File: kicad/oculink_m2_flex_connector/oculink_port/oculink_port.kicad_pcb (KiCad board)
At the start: 4 copper layers, 20.8 x 32.9 mm, 6 parts, among them J1 G14A42121B12HR, J2 Conn_01x38_Pin

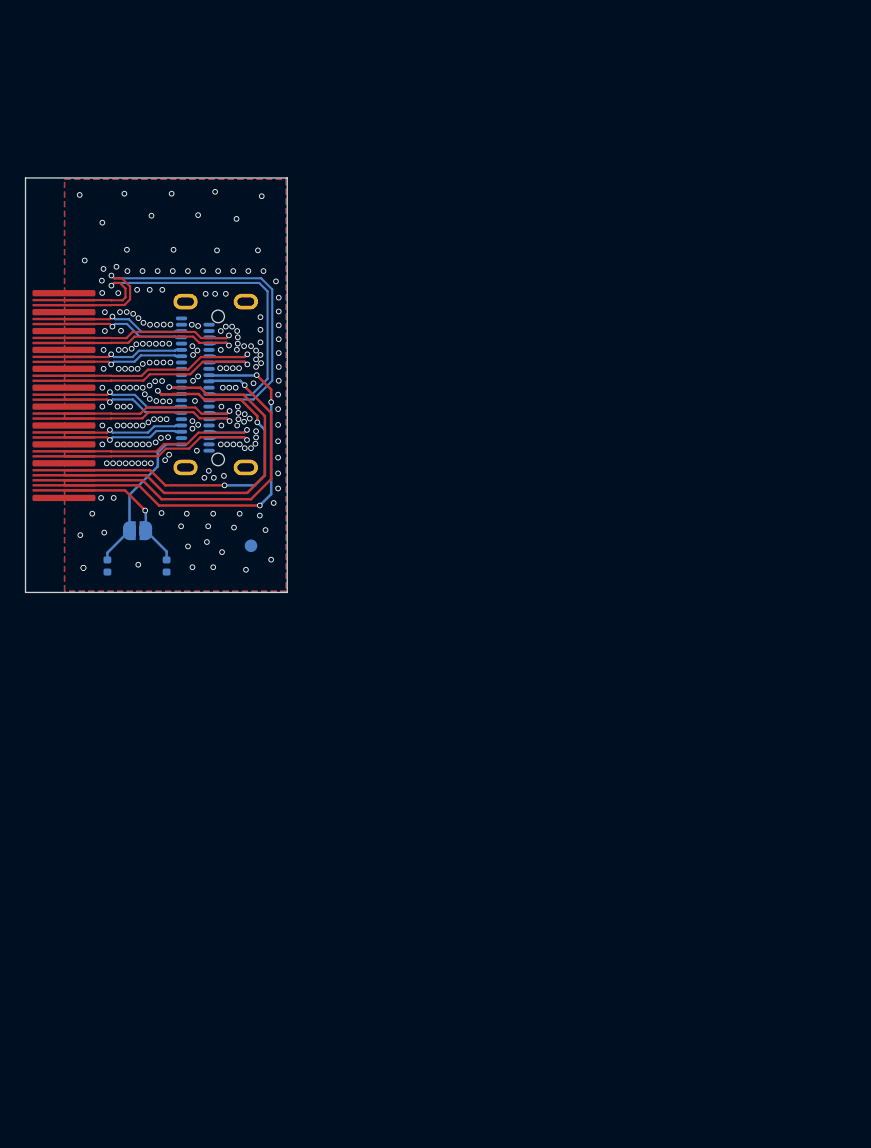
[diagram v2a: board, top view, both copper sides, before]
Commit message: Added mounting for port
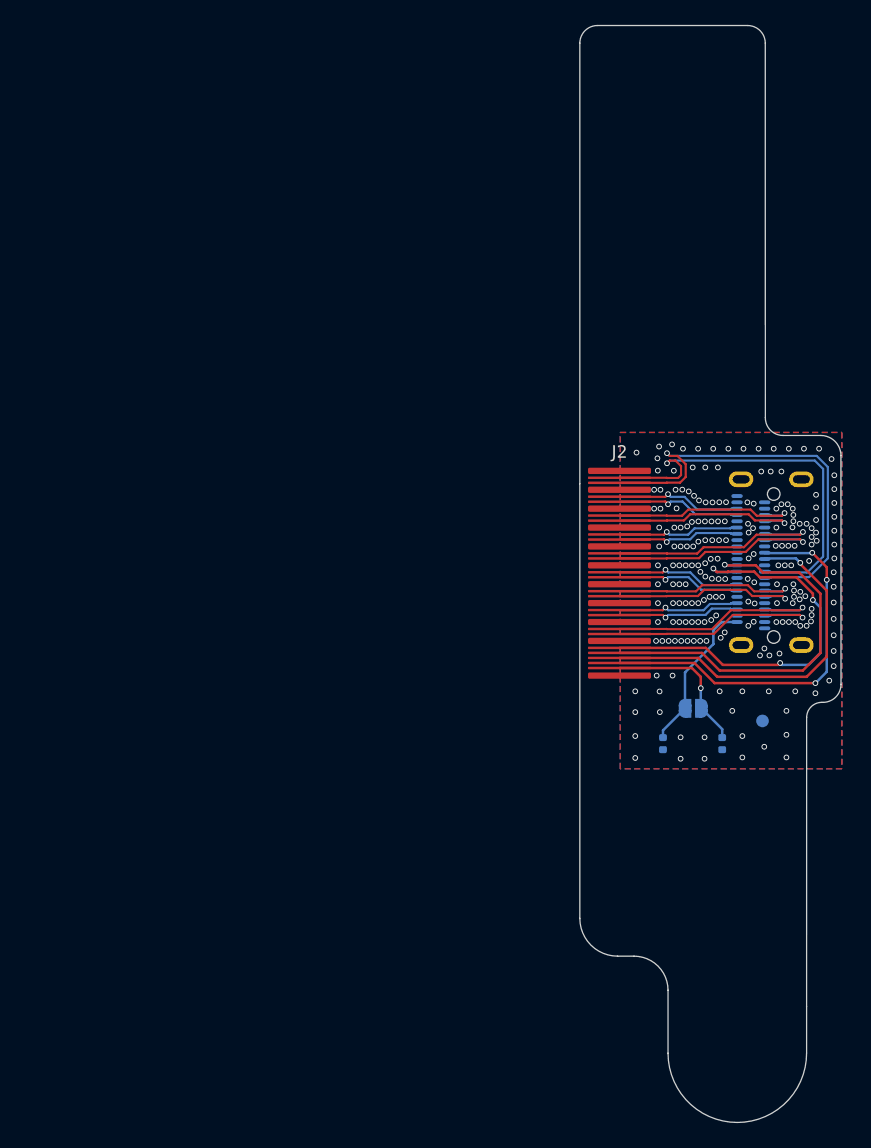
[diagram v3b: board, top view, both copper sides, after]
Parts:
- added ?: , , F.Cu at (187.1, 68.8)
- added ?: , , F.Cu at (192.2, 145.6)
- moved C1 46.3 mm to (186.3, 121.0)
- moved C5 46.3 mm to (191.0, 121.0)
- moved J1 46.3 mm to (195.1, 106.6)
- moved J2 46.3 mm to (182.8, 94.5)
- moved JP1 46.3 mm to (188.7, 118.2)
- moved TP2 42.9 mm to (194.2, 119.2)
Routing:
- net 3.3V_OPT: track 11.7 -> 12.3 mm
- net GND: vias 215 -> 205
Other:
- board size 20.8 x 32.9 mm -> 20.7 x 87.1 mm

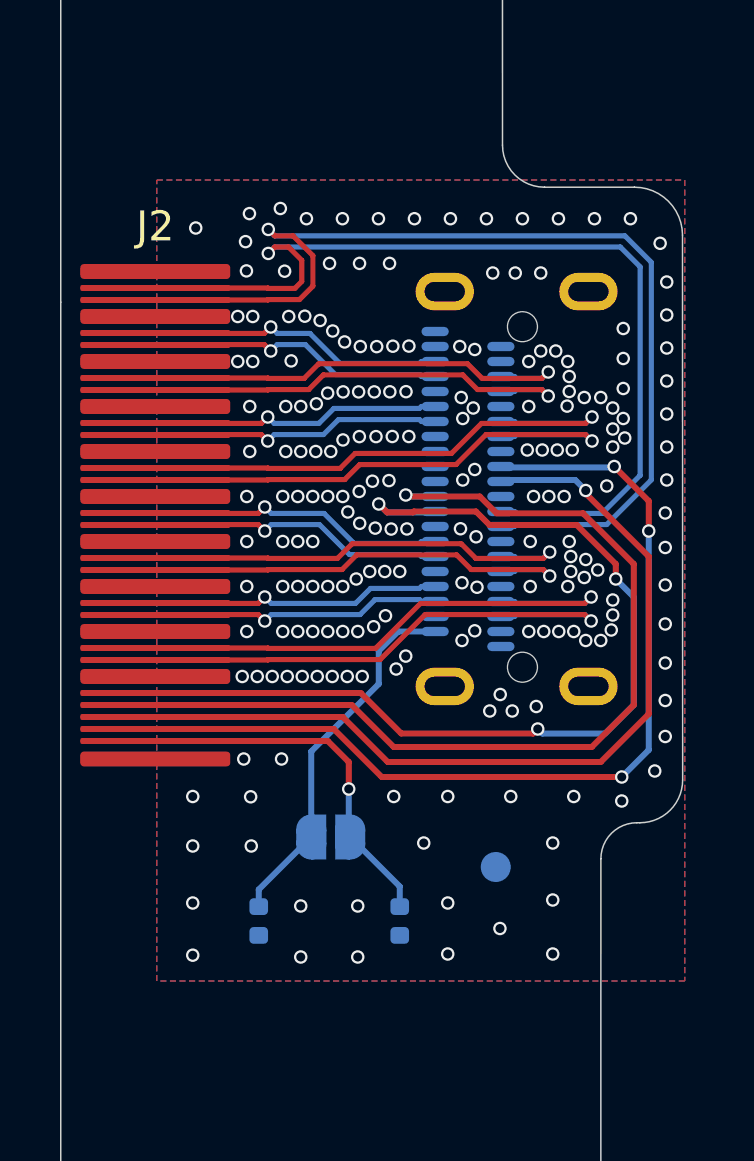
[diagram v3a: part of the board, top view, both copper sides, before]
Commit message: Shifted location of ffc connector to avoid screw mount
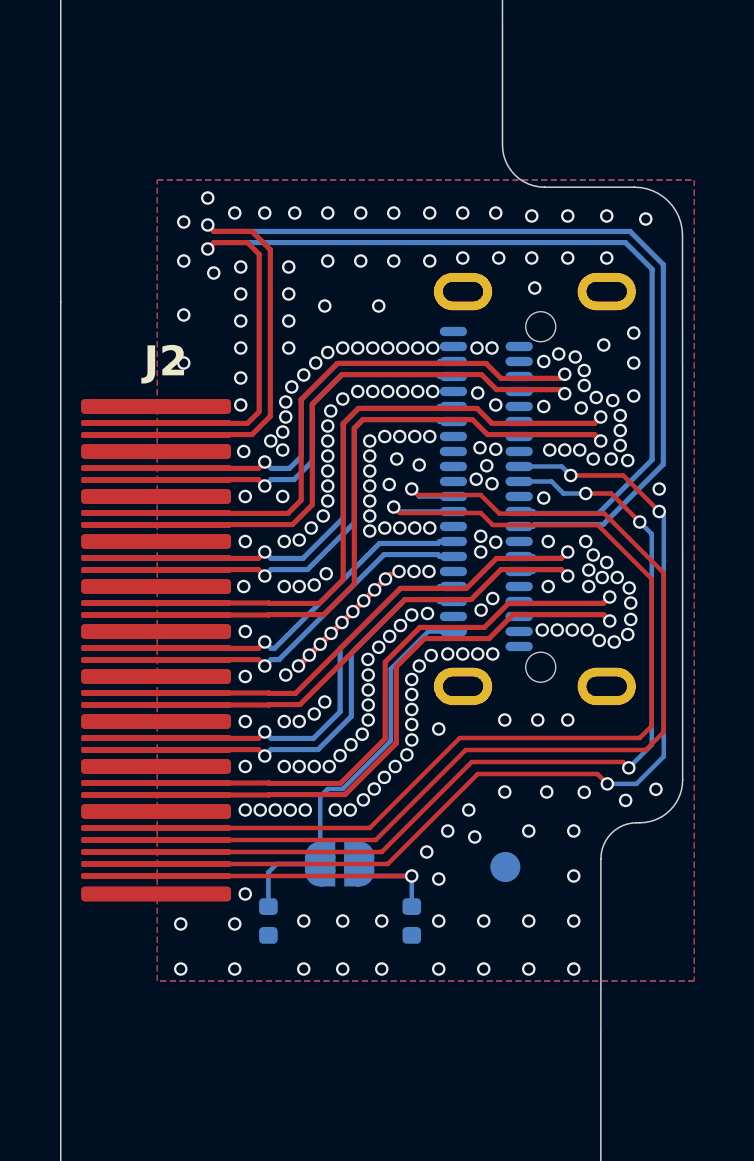
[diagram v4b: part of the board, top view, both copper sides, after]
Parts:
- moved J2 4.50 mm to (182.9, 99.0)
- moved JP1 0.95 mm to (189.0, 119.1)
- moved J1 0.61 mm to (195.7, 106.6)
- moved C5 0.40 mm to (191.4, 121.0)
- moved TP2 0.32 mm to (194.5, 119.2)
- moved C1 0.32 mm to (186.6, 121.0)
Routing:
- net CLOCK+: track 32.0 -> 37.6 mm
- net CLOCK-: track 34.4 -> 40.1 mm
- net RX1-: track 18.4 -> 23.7 mm
- net RX1+: track 18.4 -> 23.7 mm
- net TX1-: track 9.73 -> 14.0 mm
- net TX1+: track 9.73 -> 14.0 mm
- net RX0+: track 15.3 -> 19.5 mm
- net RX0-: track 15.3 -> 19.5 mm
- net RX3-: track 18.4 -> 22.3 mm
- net RX3+: track 18.4 -> 22.3 mm
- net TX3+: track 9.73 -> 13.4 mm
- net TX3-: track 9.73 -> 13.4 mm
- net PERST: track 31.4 -> 34.8 mm
- net TX0-: track 9.93 -> 12.7 mm
- net TX0+: track 9.95 -> 12.7 mm
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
